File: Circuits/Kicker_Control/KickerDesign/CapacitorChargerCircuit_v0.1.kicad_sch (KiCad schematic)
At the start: 14 parts, among them Q3 NMOS, T2 DA2034-ALD

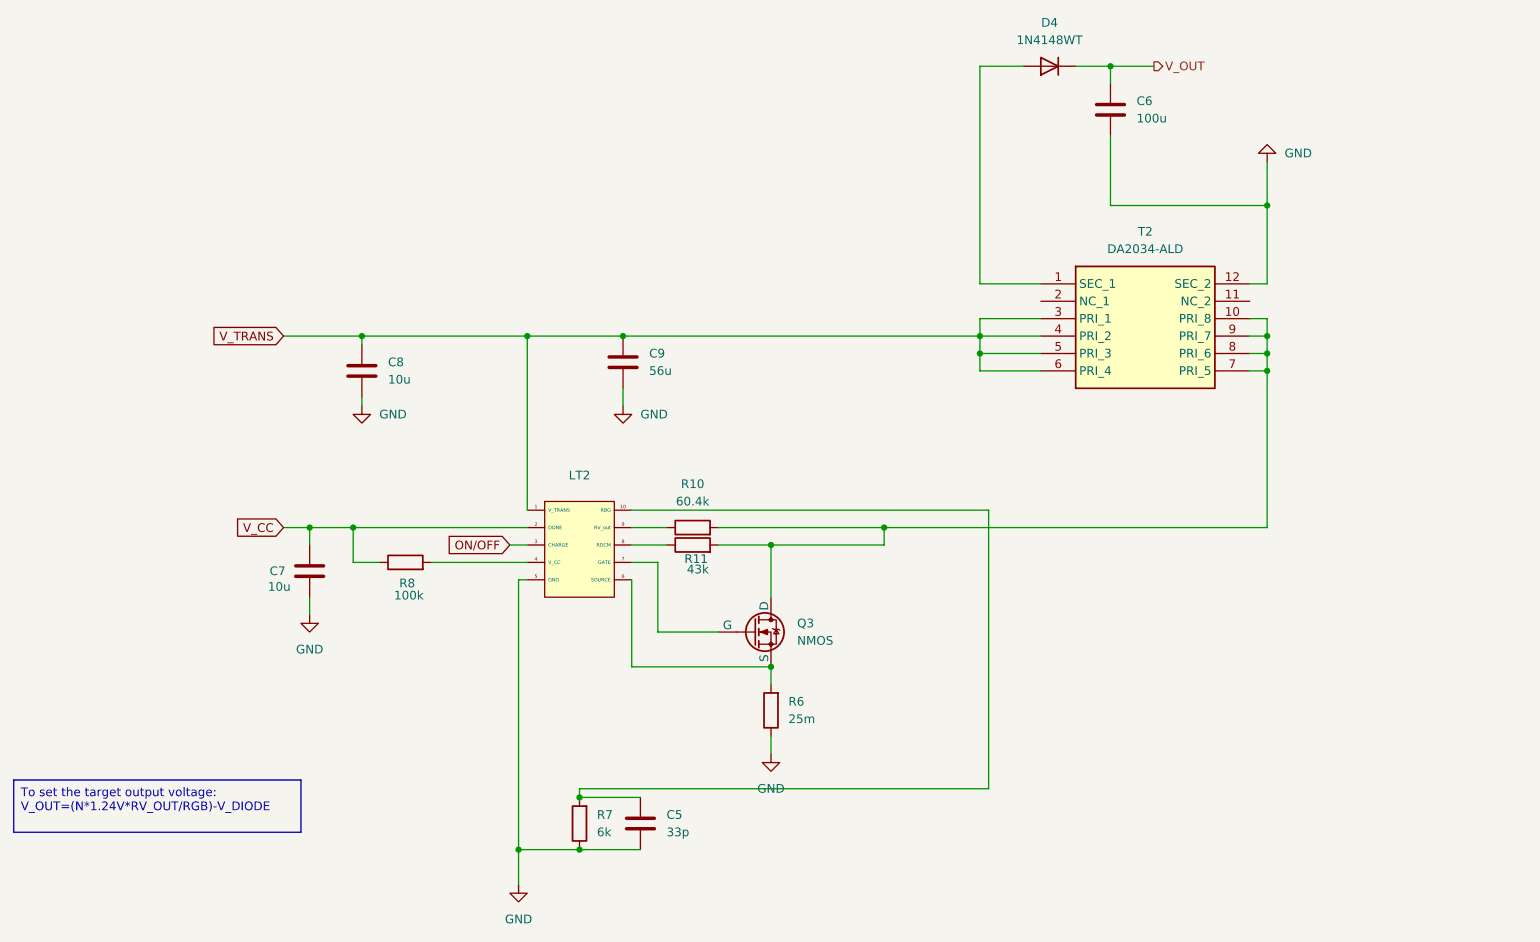
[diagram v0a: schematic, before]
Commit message: Made changes in the circuit
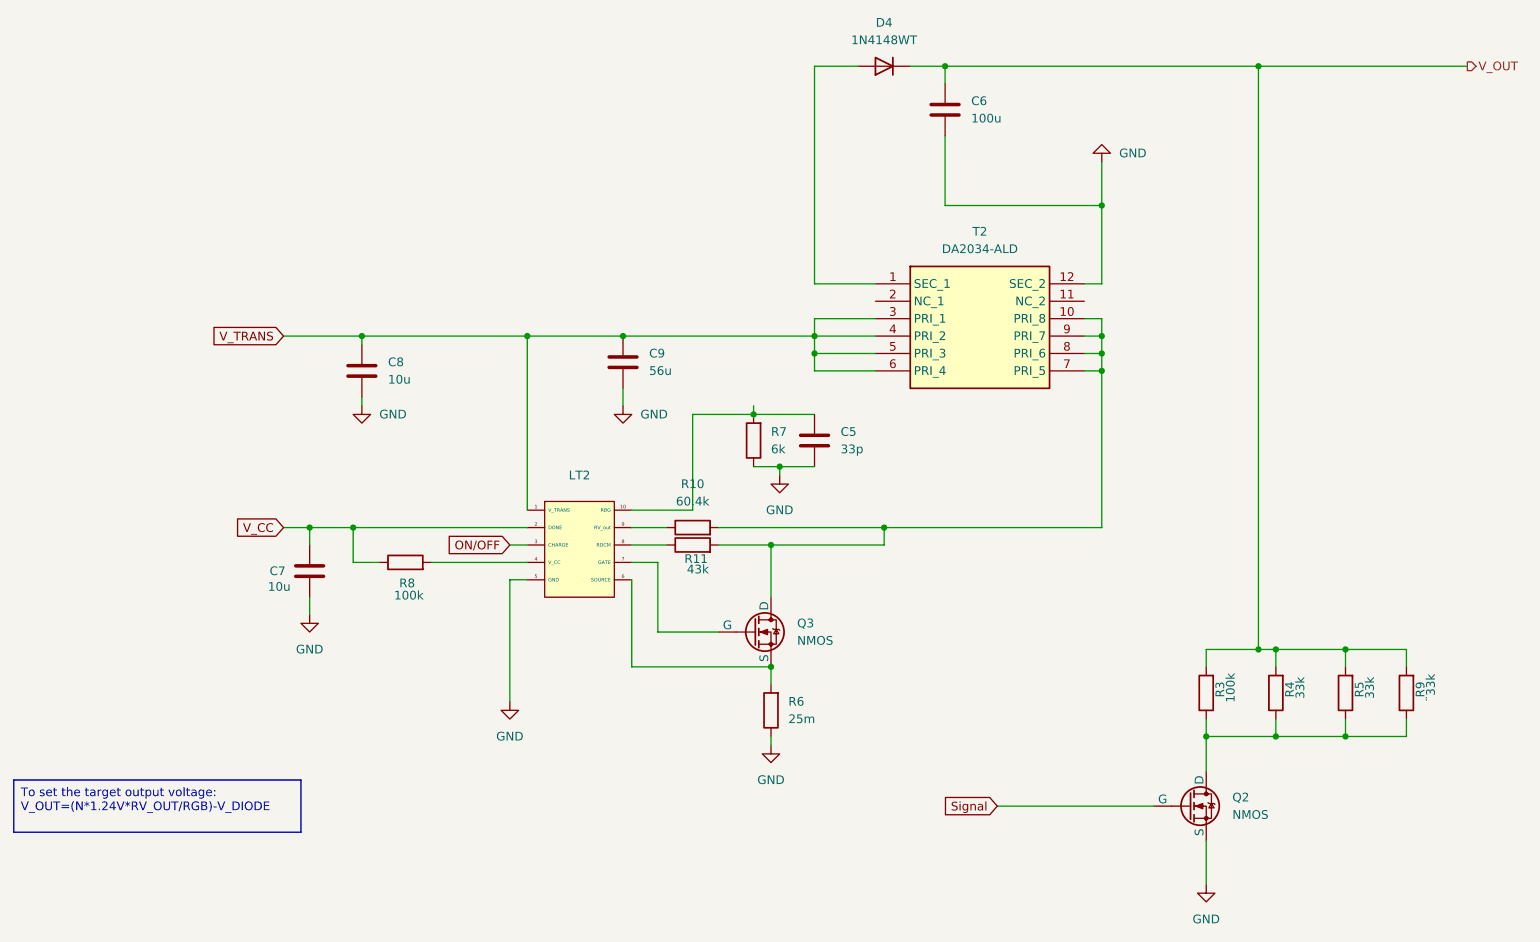
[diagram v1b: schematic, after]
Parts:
- added Q2: NMOS, symbol Simulation_SPICE:NMOS
- added R3: 100k, symbol Device:R
- added R4, R5: 33k, symbol Device:R
- added R9: ¨33k, symbol Device:R
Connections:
- net GND: now also Q2.3 (S)
- net V_OUT: now also R3.2, R4.2, R5.2, R9.2
- new net: Q2.1 (D), R3.1, R4.1, R5.1, R9.1
- new net Signal: Q2.2 (G)
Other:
- moved on the sheet: C5, C6, D4, R7, T2
